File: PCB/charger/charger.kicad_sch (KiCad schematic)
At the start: 18 parts, among them J1 Conn_01x02_Socket, J2 USB_C_Receptacle, J3 Conn_01x02_Socket, J4 Conn_01x02_Socket, J5 Conn_01x02_Socket, Q2 BSS83P, U1 MCP73831T-2ACI/OT

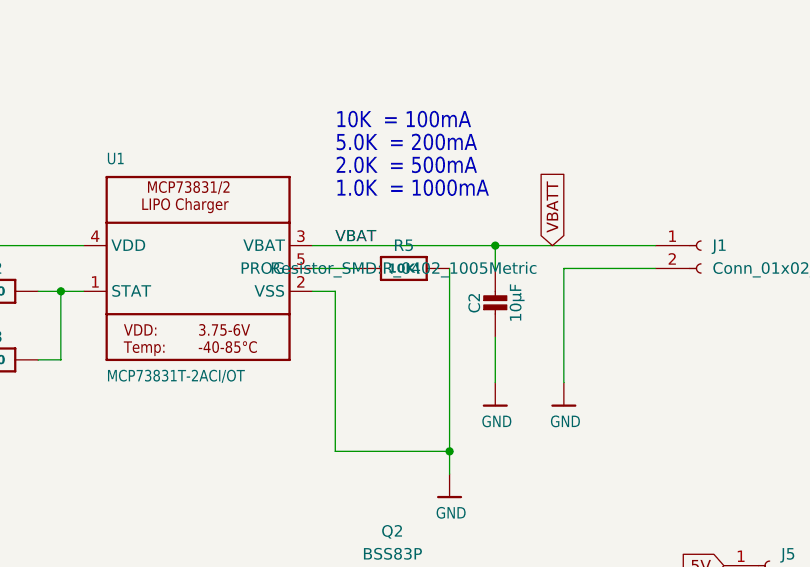
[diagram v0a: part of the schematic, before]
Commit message: idk
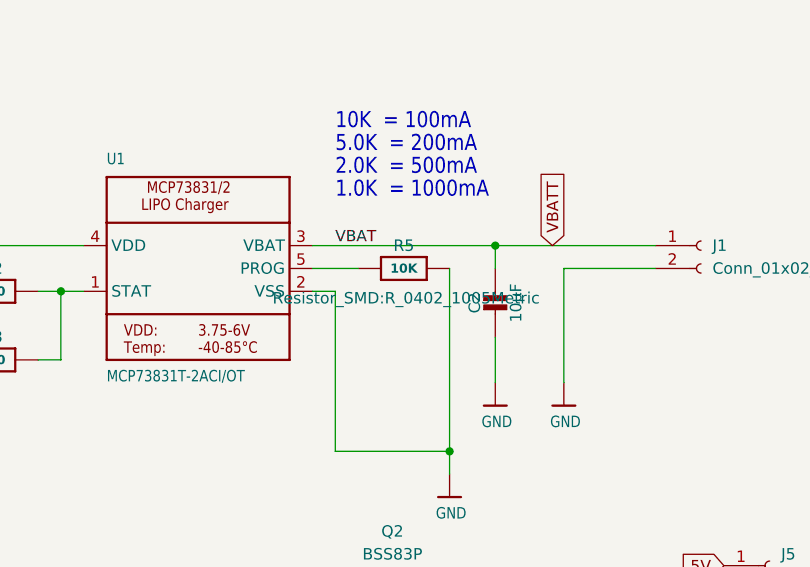
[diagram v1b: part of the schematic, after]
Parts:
- D1, D2: footprint LED_SMD:LED_0402_1005Metric -> LED_SMD:LED_0603_1608Metric
- R5: value 10K\ -> 10K
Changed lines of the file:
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@@
 			)
 		)
-		(property "Value" "10K\\"
+		(property "Value" "10K"
 			(at 217.17 68.58 0)
 			(effects
@@
 		)
 		(property "Footprint" "Resistor_SMD:R_0402_1005Metric"
-			(at 217.17 68.58 0)
+			(at 217.424 71.882 0)
 			(effects
 				(font
@@
 			)
 		)
-		(property "Footprint" "LED_SMD:LED_0402_1005Metric"
+		(property "Footprint" "LED_SMD:LED_0603_1608Metric"
 			(at 160.02 78.74 0)
 			(effects
@@
 			)
 		)
-		(property "Footprint" "LED_SMD:LED_0402_1005Metric"
+		(property "Footprint" "LED_SMD:LED_0603_1608Metric"
 			(at 160.02 71.12 0)
 			(effects
